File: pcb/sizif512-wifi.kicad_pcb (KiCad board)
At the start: 2 copper layers, 24 x 34 mm, 13 parts, among them J1 Conn_01x10, U1 AMS1117-3.3, U2 ESP-12E

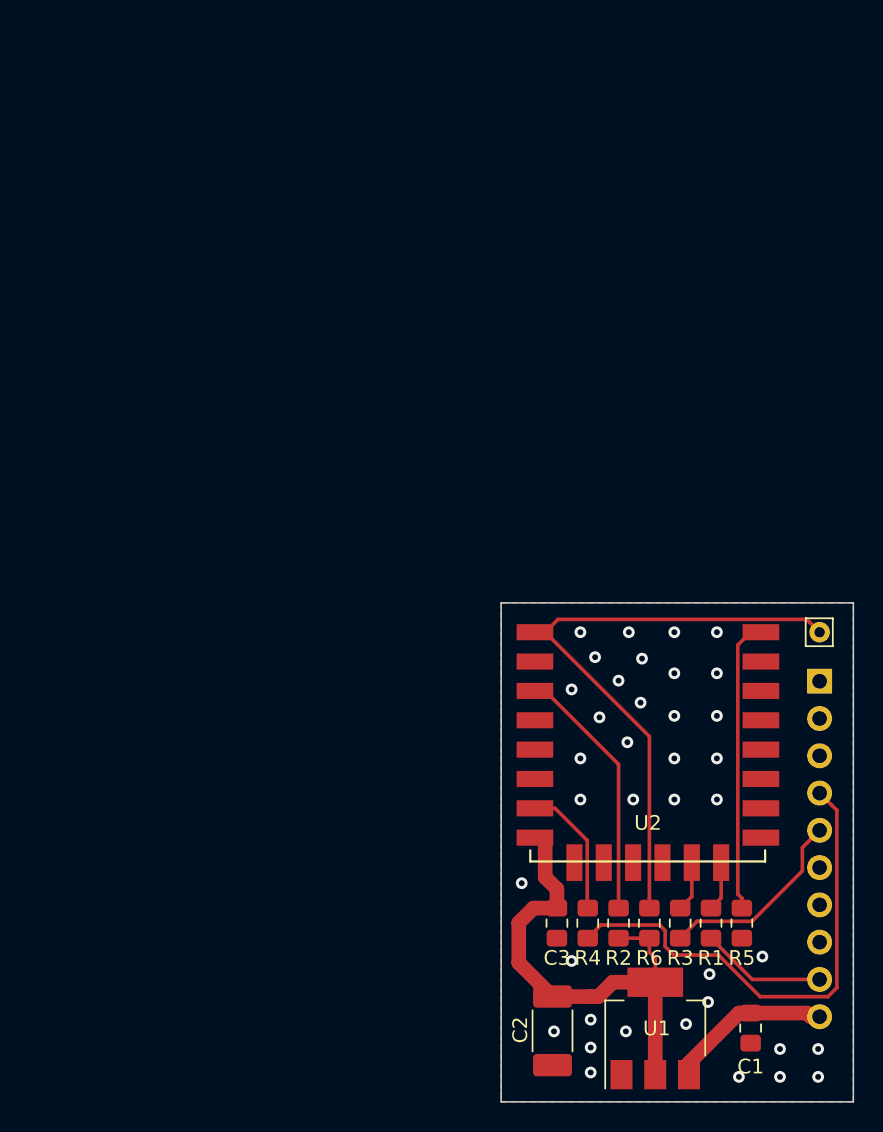
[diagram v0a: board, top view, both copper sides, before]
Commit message: import rev B files
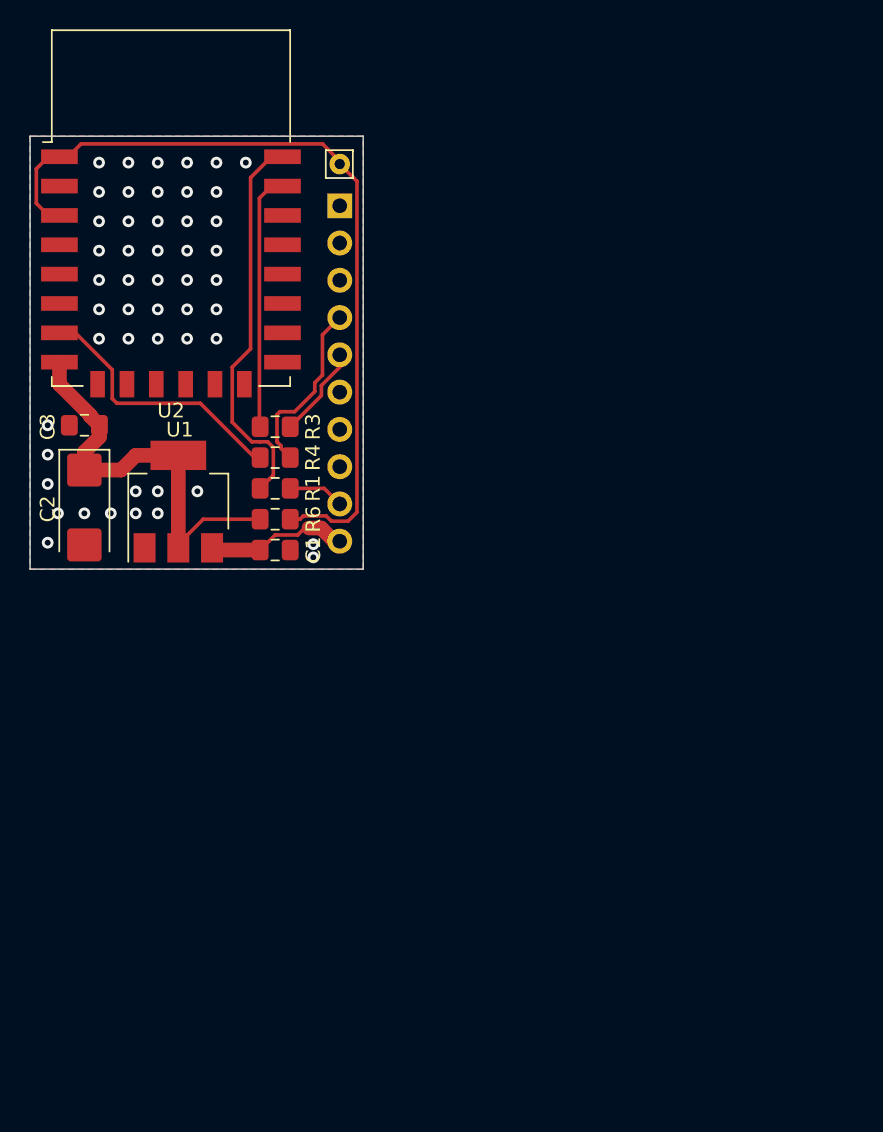
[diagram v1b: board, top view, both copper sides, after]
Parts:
- removed R2, R5: 10k, Capacitor_SMD:C_0805_2012Metric_Pad1.15x1.40mm_HandSolder
- C2: footprint Capacitor_SMD:C_2010_5025Metric_Pad1.52x2.65mm_HandSolder -> Capacitor_Tantalum_SMD:CP_EIA-6032-15_Kemet-U_Pad2.25x2.35mm_HandSolder
- R1: value 560 -> 47
- U2: footprint ESP8266:ESP-12E_SMD -> RF_Module:ESP-12E
- moved U1 48.4 mm to (146.5, 106.6)
- moved C2 47.8 mm to (140.1, 107.0)
- moved C3 46.8 mm to (140.1, 101.4), turned to 180 degrees
- moved J1 46.0 mm to (157.5, 86.4)
- moved C1 45.9 mm to (153.1, 109.9), turned to 0 degrees
- moved TP1 45.7 mm to (157.5, 83.6)
- moved R3 43.7 mm to (153.1, 101.5), turned to 0 degrees
- moved R1 41.9 mm to (153.1, 105.7), turned to 0 degrees
- moved U2 38.5 mm to (146.0, 86.6)
- moved R4 38.2 mm to (153.1, 103.6), turned to 0 degrees
- moved R6 37.5 mm to (153.1, 107.8), turned to 180 degrees
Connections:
- U2 pad 16: Net-(R5-Pad2) -> GND
- U2 pad 3: Net-(R2-Pad1) -> Net-(R6-Pad1)
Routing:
- net Net-(R1-Pad1): track 4.09 -> 26.6 mm
- net CTS: track 34.0 -> 12.3 mm
- net Net-(R5-Pad2): track 19.3 -> 0.00 mm
- net Net-(R2-Pad1): track 16.9 -> 0.00 mm
- net Net-(R6-Pad1): track 41.2 -> 55.1 mm
- net Net-(R3-Pad1): track 4.13 -> 17.5 mm
- net Net-(R4-Pad1): track 8.40 -> 18.4 mm
- net TX: track 13.5 -> 6.30 mm
- net RX: track 8.56 -> 3.81 mm
- net +3V3: track 33.1 -> 28.5 mm
- net +5V: track 11.2 -> 9.76 mm
- net GND: vias 38 -> 50
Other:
- board size 24 x 34 mm -> 22.7 x 29.5 mm
- board text added: "SIZIF-512 WiFi Module Rev.B"
- board text removed: "SIZIF-512 WiFi Module Rev.A"

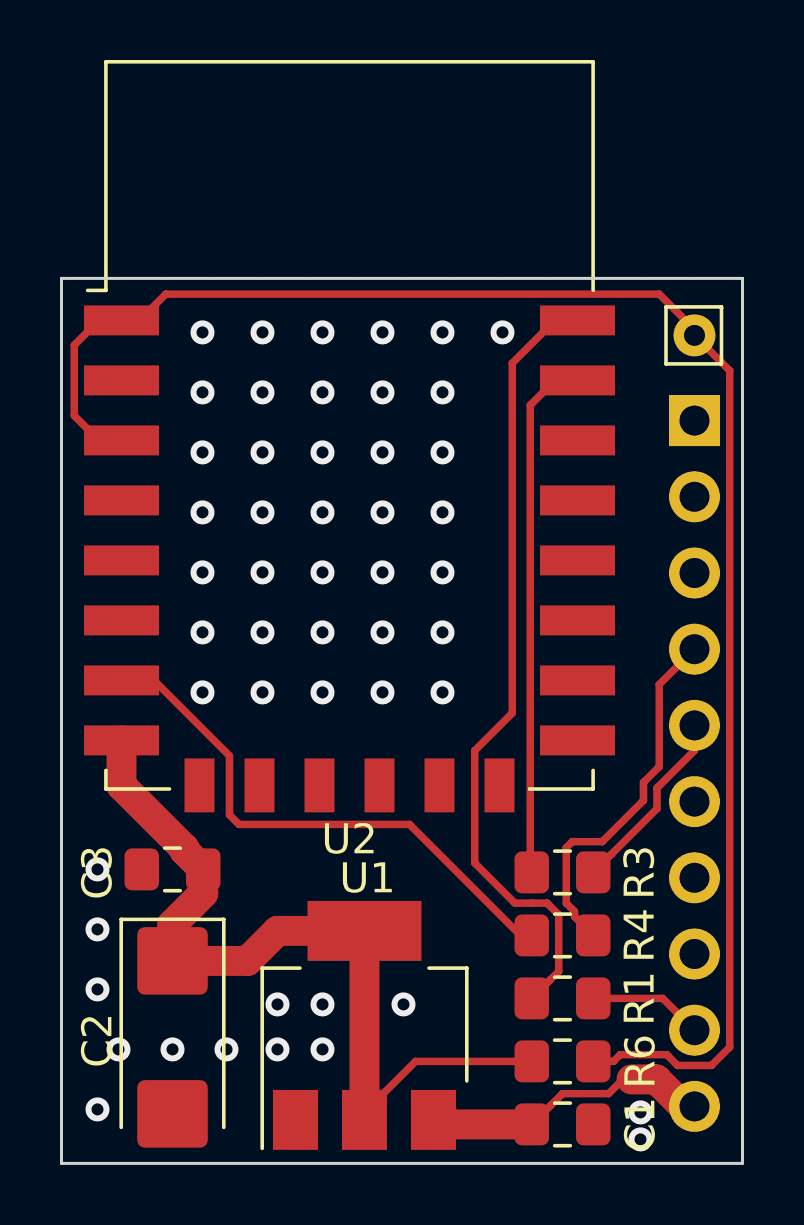
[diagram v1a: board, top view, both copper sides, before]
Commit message: import rev C files
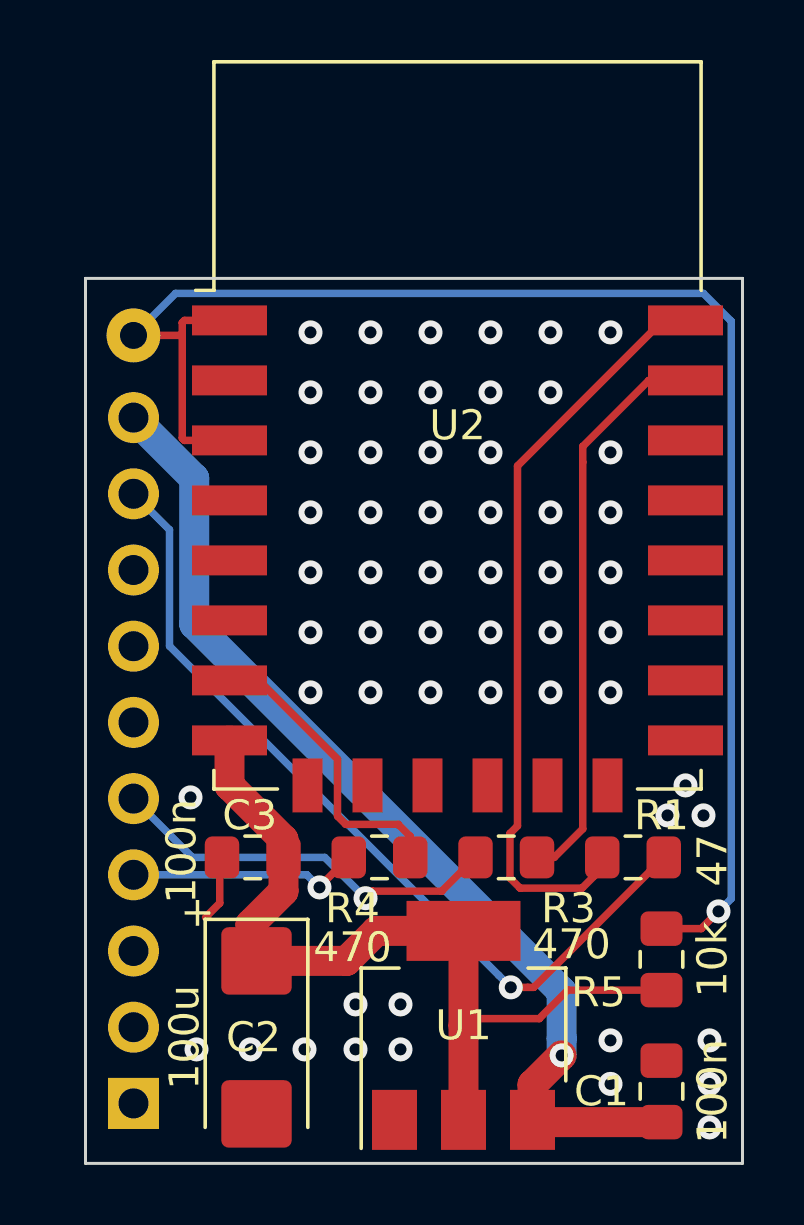
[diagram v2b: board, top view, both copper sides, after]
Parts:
- removed R6: 10k, Capacitor_SMD:C_0805_2012Metric_Pad1.15x1.40mm_HandSolder
- added R5: 10k, Capacitor_SMD:C_0805_2012Metric_Pad1.15x1.40mm_HandSolder, F.Cu at (156.4, 104.4)
- R3, R4: value 560 -> 470
- TP1: footprint Connector_Pin:Pin_D0.7mm_L6.5mm_W1.8mm_FlatFork -> Connector_Pin:Pin_D0.9mm_L10.0mm_W2.4mm_FlatFork; moved to B.Cu
- moved J1 29.5 mm to (138.8, 109.2), turned to 0 degrees
- moved TP1 18.7 mm to (138.8, 83.6)
- moved R4 6.63 mm to (147.0, 101.0), turned to 180 degrees
- moved R1 5.25 mm to (155.4, 101.0)
- moved U2 3.60 mm to (149.6, 86.6)
- moved C1 3.48 mm to (156.4, 108.8), turned to 90 degrees
- moved U1 3.30 mm to (149.8, 106.6)
- moved C2 2.80 mm to (142.9, 107.0)
- moved C3 2.70 mm to (142.8, 101.0)
- moved R3 1.94 mm to (151.2, 101.0), turned to 180 degrees
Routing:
- net RX: track 3.81 -> 28.6 mm, vias 0 -> 1
- net +5V: track 9.76 -> 34.1 mm, vias 0 -> 1
- net Net-(R4-Pad1): track 18.4 -> 9.99 mm
- net TX: track 6.30 -> 13.3 mm, vias 0 -> 1
- net CTS: track 12.3 -> 7.78 mm, vias 0 -> 1
- net Net-(R5-Pad1): track 55.1 -> 53.1 mm, vias 0 -> 1
- net GND: track 0.00 -> 1.80 mm, vias 50 -> 56
- net Net-(R3-Pad1): track 17.5 -> 19.0 mm
- net Net-(R1-Pad1): track 26.6 -> 25.2 mm
- net +3V3: track 28.5 -> 29.3 mm
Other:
- board size 22.7 x 29.5 mm -> 21.9 x 29.5 mm
- board text added: "Sizif-512 WiFi Module Rev.C"
- board text removed: "SIZIF-512 WiFi Module Rev.B"
